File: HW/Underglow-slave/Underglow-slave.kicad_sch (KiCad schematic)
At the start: 8 parts, among them J1 Debug_header, U1 CH572Q, Y1 Crystal

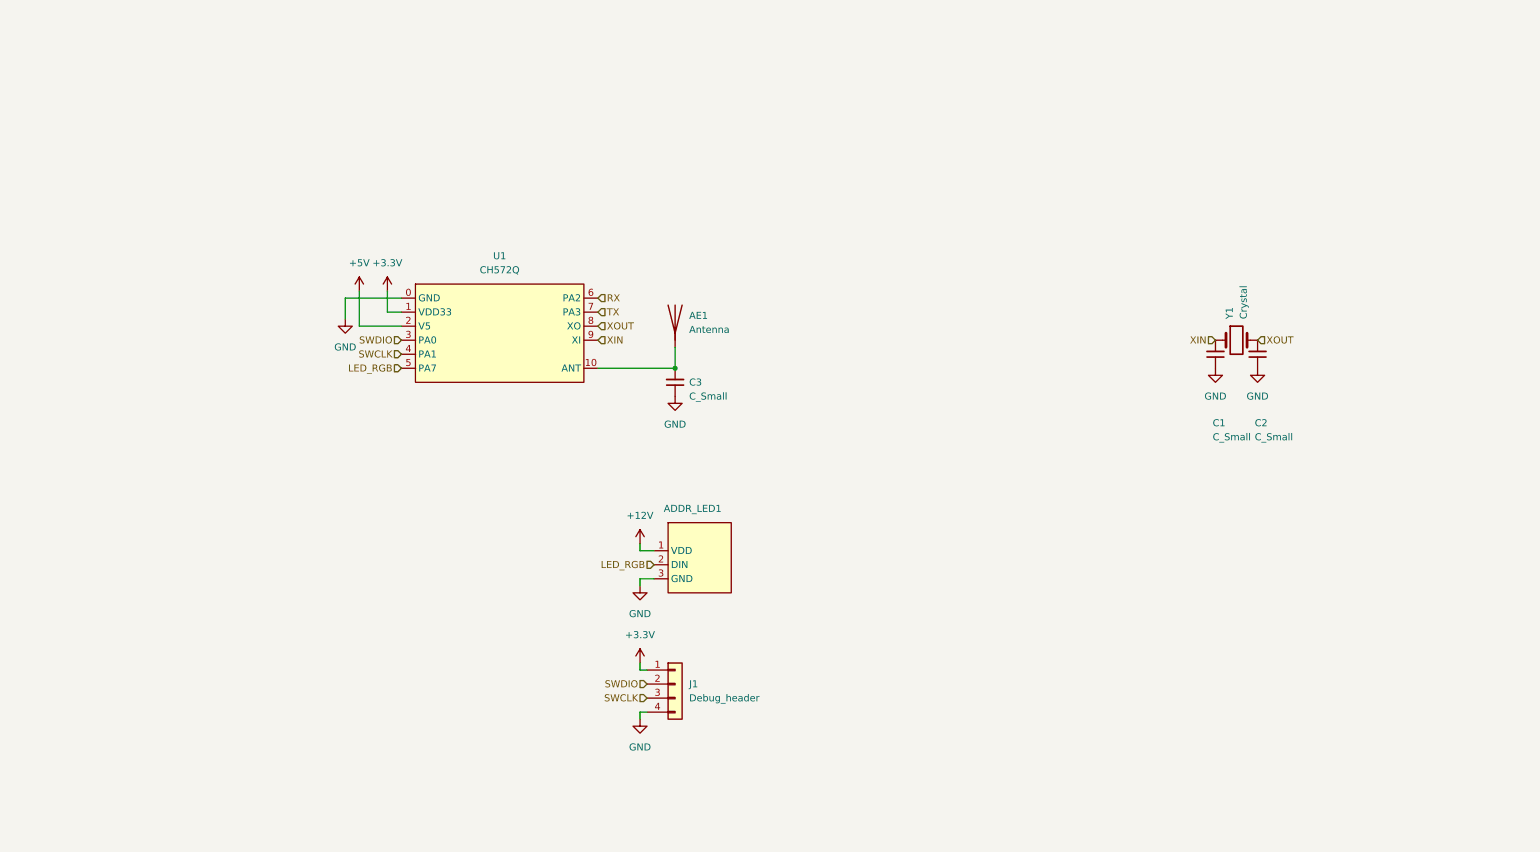
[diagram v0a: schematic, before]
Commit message: claude did something
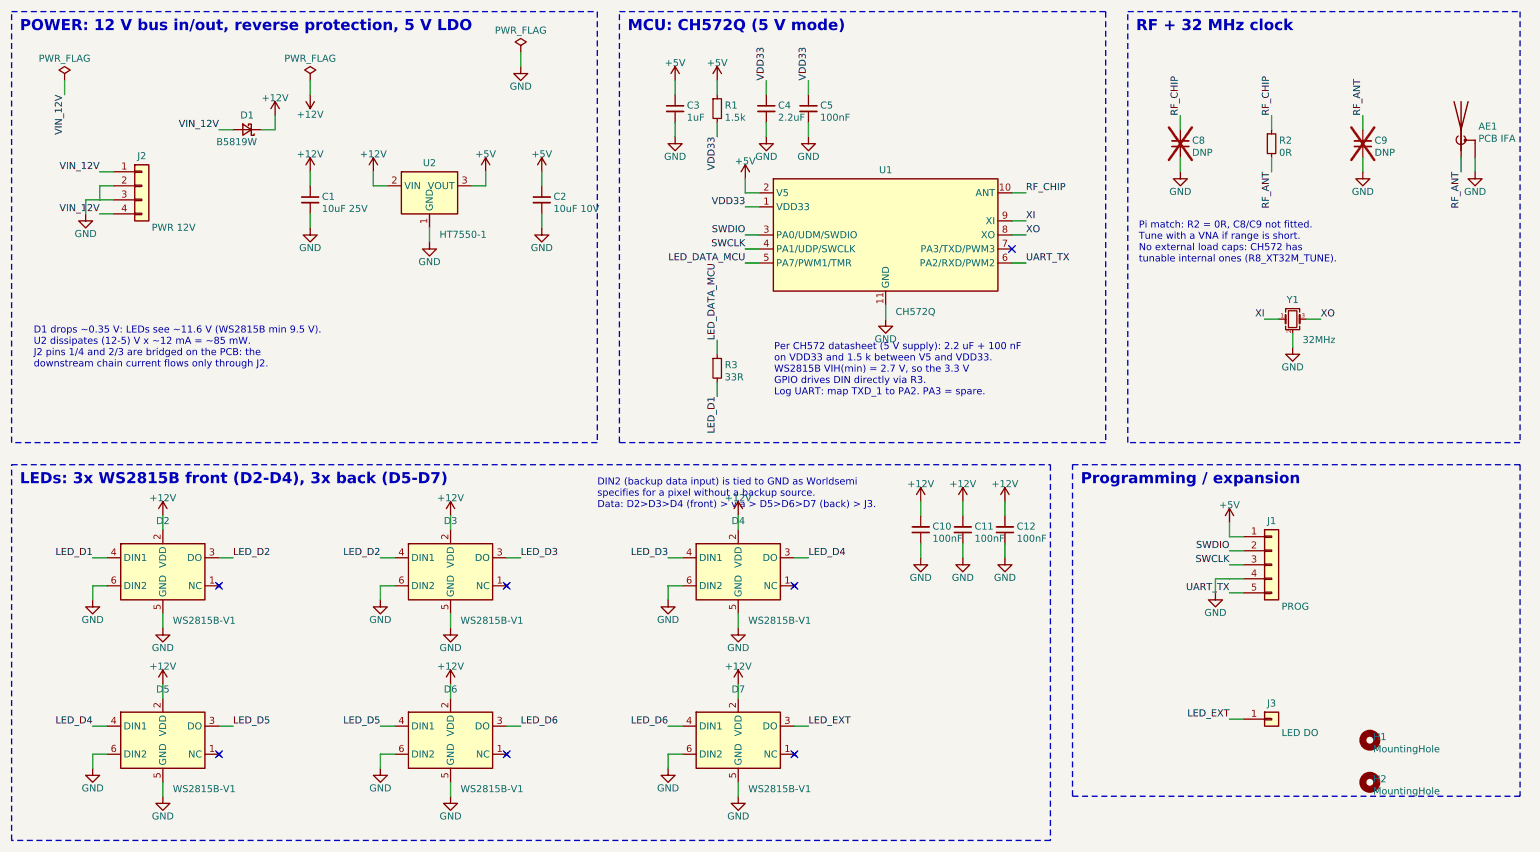
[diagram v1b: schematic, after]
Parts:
- removed ADDR_LED1: (no value), Mylib:Addressable_led_adapter_10mm, symbol Mylib:LED_addr_adapter
- removed AE1: Antenna, RF_Antenna:Texas_SWRA117D_2.4GHz_Right, symbol Device:Antenna
- removed J1: Debug_header, symbol Connector_Generic:Conn_01x04
- removed U1: CH572Q, Package_DFN_QFN:DFN-10-1EP_2.6x2.6mm_P0.5mm_EP1.3x2.2mm, symbol Mylib:CH572
- removed Y1: Crystal, symbol Device:Crystal
- added AE1: PCB IFA, RF_Antenna:Texas_SWRA117D_2.4GHz_Right, symbol Device:Antenna_Shield
- added C10, C11, C12, C5: 100nF, Capacitor_SMD:C_0402_1005Metric, symbol Device:C_Small
- added C4: 2.2uF, Capacitor_SMD:C_0402_1005Metric, symbol Device:C_Small
- added C8, C9: DNP, Capacitor_SMD:C_0402_1005Metric, symbol Device:C_Small
- added D1: B5819W, Diode_SMD:D_SOD-123, symbol Device:D_Schottky_Small
- added D2, D3, D4, D5, D6, D7: WS2815B-V1, LED_SMD:LED_WS2812_PLCC6_5.0x5.0mm_P1.6mm, symbol TreeGlow:WS2815B
- added H1, H2: MountingHole, MountingHole:MountingHole_2.2mm_M2, symbol Mechanical:MountingHole
- added J1: PROG, TreeGlow:ProgPads_1x05_P2.54mm, symbol Connector_Generic:Conn_01x05
- added J2: PWR 12V, Connector_Wire:SolderWire-0.75sqmm_1x04_P4.8mm_D1.25mm_OD2.3mm, symbol Connector_Generic:Conn_01x04
- added J3: LED DO, TestPoint:TestPoint_Pad_D1.5mm, symbol Connector_Generic:Conn_01x01
- added R1: 1.5k, Capacitor_SMD:C_0402_1005Metric, symbol Device:R_Small
- added R2: 0R, Capacitor_SMD:C_0402_1005Metric, symbol Device:R_Small
- added R3: 33R, Capacitor_SMD:C_0402_1005Metric, symbol Device:R_Small
- added U1: CH572Q, Package_DFN_QFN:DFN-10-1EP_3x3mm_P0.5mm_EP1.7x2.5mm, symbol TreeGlow:CH572Q
- added U2: HT7550-1, Package_TO_SOT_SMD:SOT-89-3, symbol Regulator_Linear:HT75xx-1-SOT89
- added Y1: 32MHz, Crystal:Crystal_SMD_3225-4Pin_3.2x2.5mm, symbol Device:Crystal_GND24_Small
- C1: value C_Small -> 10uF 25V; footprint (none) -> Capacitor_SMD:C_0805_2012Metric; LCSC (none) -> C15850
- C2: value C_Small -> 10uF 10V; footprint (none) -> Capacitor_SMD:C_0603_1608Metric; LCSC (none) -> C19702
- C3: value C_Small -> 1uF; footprint (none) -> Capacitor_SMD:C_0402_1005Metric; LCSC (none) -> C52923
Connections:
- net XIN is gone; now on net GND: C1.2
- net XOUT is gone; now on net GND: C2.2
- net +12V: now also C1.1, C10.1, C11.1, C12.1, D1.1 (K), D2.2 (VDD), D3.2 (VDD), D4.2 (VDD), D5.2 (VDD), D6.2 (VDD), D7.2 (VDD), U2.2 (VIN)
- net +5V: now also C2.1, C3.1, J1.1 (Pin_1), R1.1, U1.2 (V5), U2.3 (VOUT)
- net GND: now also C3.2, AE1.2 (Shield), C10.2, C11.2, C12.2, C4.2, C5.2, C8.2, C9.2, D2.5 (GND), D2.6 (DIN2), D3.5 (GND), D3.6 (DIN2), D4.5 (GND), D4.6 (DIN2), D5.5 (GND), D5.6 (DIN2), D6.5 (GND), D6.6 (DIN2), D7.5 (GND), D7.6 (DIN2), J1.4 (Pin_4), J2.2 (Pin_2), J2.3 (Pin_3), U1.11 (GND), U2.1 (GND), Y1.2 (G), Y1.4 (G); no longer C1.1, C2.1, C3.1
- net SWCLK: now also J1.3 (Pin_3), U1.4 (PA1/UDP/SWCLK)
- net SWDIO: now also J1.2 (Pin_2), U1.3 (PA0/UDM/SWDIO)
- new net LED_D1: D2.4 (DIN1), R3.2
- new net LED_D2: D2.3 (DO), D3.4 (DIN1)
- new net LED_D3: D3.3 (DO), D4.4 (DIN1)
- new net LED_D4: D4.3 (DO), D5.4 (DIN1)
- new net LED_D5: D5.3 (DO), D6.4 (DIN1)
- new net LED_D6: D6.3 (DO), D7.4 (DIN1)
- new net LED_DATA_MCU: R3.1, U1.5 (PA7/PWM1/TMR)
- new net LED_EXT: D7.3 (DO), J3.1 (Pin_1)
- new net RF_ANT: AE1.1 (A), C9.1, R2.2
- new net RF_CHIP: C8.1, R2.1, U1.10 (ANT)
- new net UART_TX: J1.5 (Pin_5), U1.6 (PA2/RXD/PWM2)
- new net VDD33: C4.1, C5.1, R1.2, U1.1 (VDD33)
- new net VIN_12V: D1.2 (A), J2.1 (Pin_1), J2.4 (Pin_4)
- new net XI: U1.9 (XI), Y1.1
- new net XO: U1.8 (XO), Y1.3
- no-connect marks 0 -> 7
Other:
- note added: "D1 drops ~0.35 V: LEDs see ~11.6 V (WS2815B min 9.5 V). U2 dissipates (12-5) V x ~12 mA = ~85 mW. J2 pins 1/4 and 2/3 are bridged on the PCB: the downstream chain current flows only through J2."
- note added: "DIN2 (backup data input) is tied to GND as Worldsemi specifies for a pixel without a backup source. Data: D2>D3>D4 (front) > via > D5>D6>D7 (back) > J3."
- note added: "LEDs: 3x WS2815B front (D2-D4), 3x back (D5-D7)"
- note added: "MCU: CH572Q (5 V mode)"
- note added: "POWER: 12 V bus in/out, reverse protection, 5 V LDO"
- note added: "Per CH572 datasheet (5 V supply): 2.2 uF + 100 nF on VDD33 and 1.5 k between V5 and VDD33. WS2815B VIH(min) = 2.7 V, so the 3.3 V GPIO drives DIN directly via R3. Log UART: map TXD_1 to PA2. PA3 = spare."
- note added: "Pi match: R2 = 0R, C8/C9 not fitted. Tune with a VNA if range is short. No external load caps: CH572 has tunable internal ones (R8_XT32M_TUNE)."
- note added: "Programming / expansion"
- note added: "RF + 32 MHz clock"
- title: (none) -> TreeGlow node (CH572Q + 6x WS2815B)
